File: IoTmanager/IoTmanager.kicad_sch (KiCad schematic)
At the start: 42 parts, among them J1 Program-connector, K1 ZC32F-012-HS3-copy, K2 ZC32F-012-HS3-copy, K3 ZC32F-012-HS3-copy, K4 ZC32F-012-HS3-copy, Q1 BC817, Q2 BC817, Q3 BC817, Q4 BC817, U1 NodeMCU_1.0_(ESP-12E), U2 ESP-12F, U3 TSOP23xx, U4 Mini360, U5 PJ-320A, U6 AMS1117-3.3

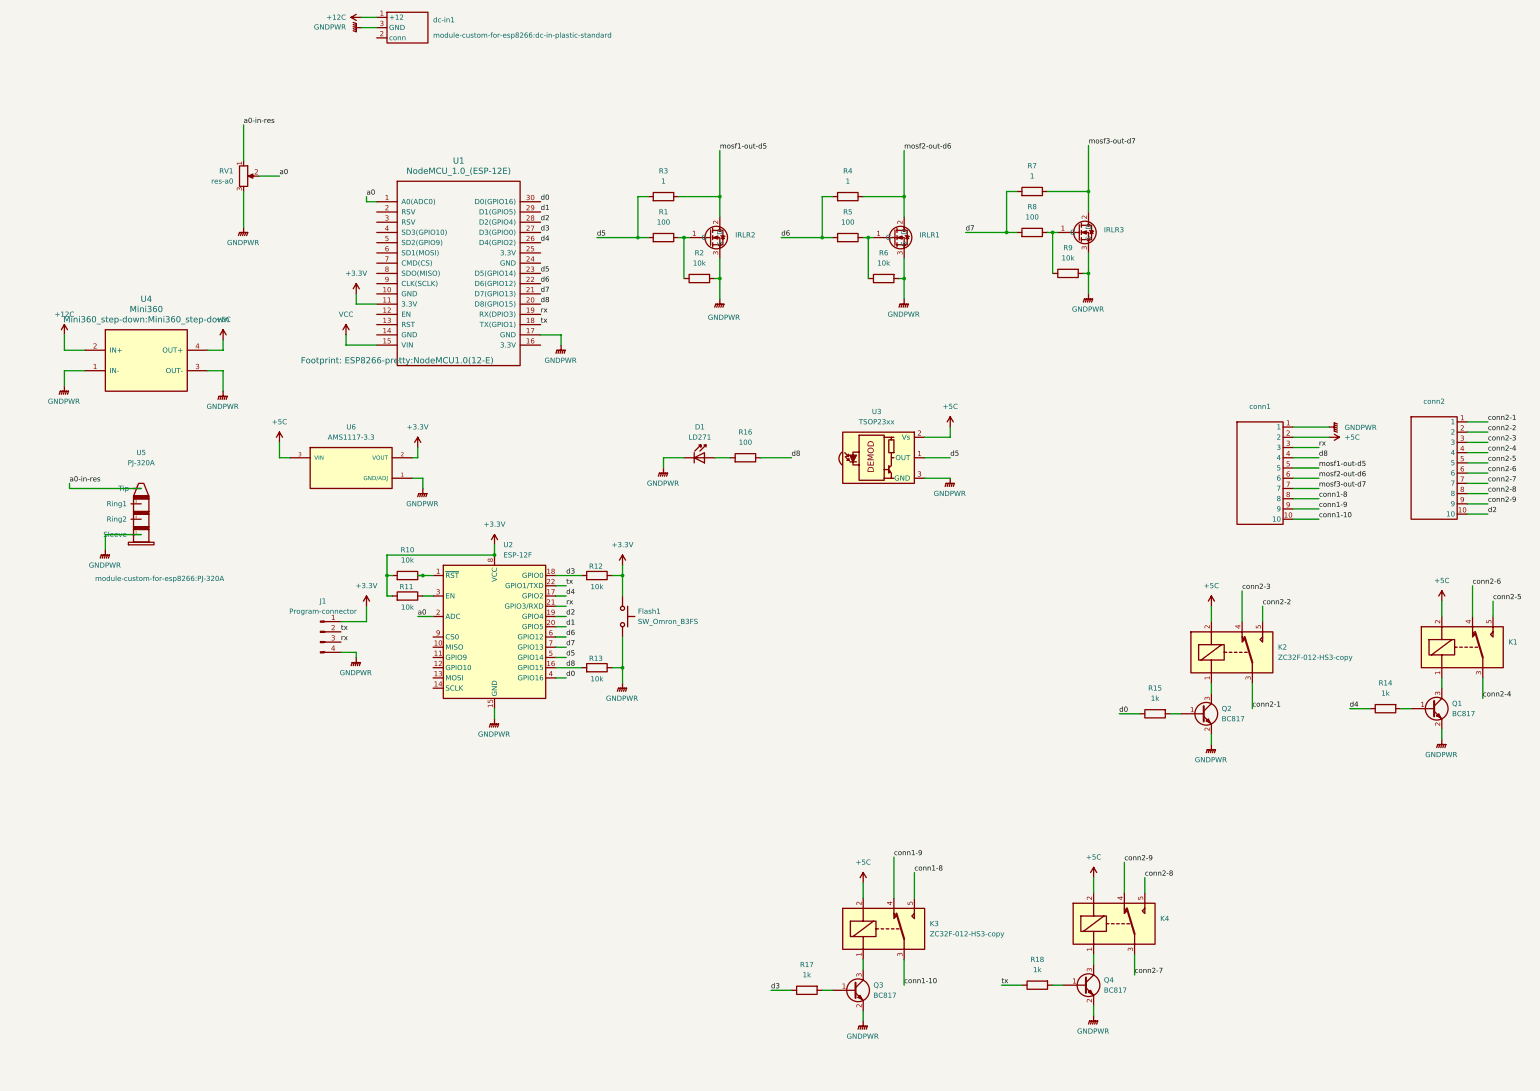
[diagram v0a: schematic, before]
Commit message: 123
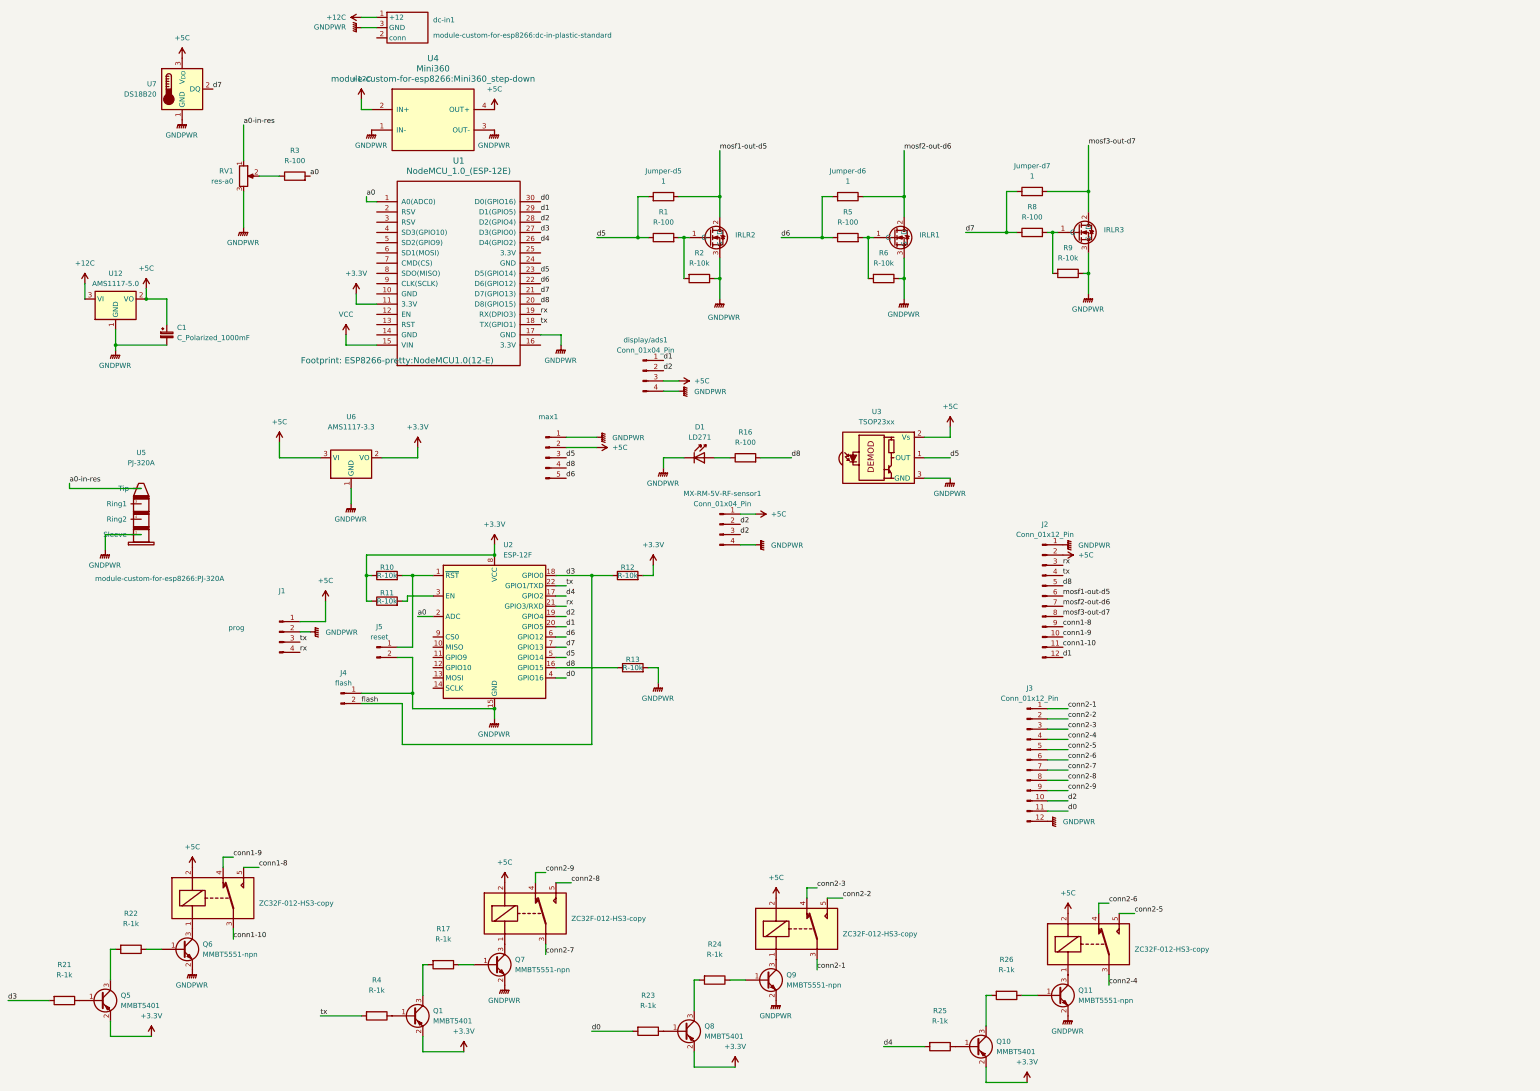
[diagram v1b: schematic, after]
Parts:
- removed Flash1: SW_Omron_B3FS, Button_Switch_SMD:SW_SPST_Omron_B3FS-100xP, symbol Switch:SW_Omron_B3FS
- removed K1, K2, K4: ZC32F-012-HS3-copy, module-custom-for-esp8266:ZC32F-012-HS3, symbol models:ZC32F-012-HS3-copy
- removed Q1, Q2, Q3, Q4: BC817, Package_TO_SOT_SMD:SOT-23, symbol Transistor_BJT:BC817
- removed R10: 10k, Resistor_SMD:R_0805_2012Metric, symbol resistor:R-base
- removed R14, R15, R17, R18: 1k, Resistor_SMD:R_0805_2012Metric, symbol resistor:R-base
- removed conn1, conn2: ~, module-custom-for-esp8266:connector-10, symbol models:CONNECTOR-10
- added C1: C_Polarized_1000mF, Capacitor_THT:CP_Radial_D10.0mm_P3.50mm, symbol resistor:C_Polarized_Small
- added J2, J3: Conn_01x12_Pin, module-custom-for-esp8266:connector-12-green-mini, symbol Connector:Conn_01x12_Pin
- added J4: flash, Connector_PinHeader_2.54mm:PinHeader_1x02_P2.54mm_Vertical, symbol Connector:Conn_01x02_Pin
- added J5: reset, Connector_PinHeader_2.54mm:PinHeader_1x02_P2.54mm_Vertical, symbol Connector:Conn_01x02_Pin
- added K5, K6, K7: ZC32F-012-HS3-copy, module-custom-for-esp8266:ZC32F-012-HS3, symbol models:ZC32F-012-HS3-copy
- added MX-RM-5V-RF-sensor1: Conn_01x04_Pin, module-custom-for-esp8266:RF_Receiver_433_MHz, symbol Connector:Conn_01x04_Pin
- added Q1, Q10, Q5, Q8: MMBT5401, Package_TO_SOT_SMD:SOT-23, symbol models:MMBT5401-pnp
- added Q11, Q6, Q7, Q9: MMBT5551-npn, Package_TO_SOT_SMD:SOT-23, symbol models:MMBT5551-npn
- added R10: R-10k, Resistor_SMD:R_0805_2012Metric, symbol models:R-10k
- added R17, R21, R22, R23, R24, R25, R26, R4: R-1k, Resistor_SMD:R_0805_2012Metric, symbol models:R-1k
- added R3: R-100, Resistor_SMD:R_0805_2012Metric, symbol models:R-100
- added U12: AMS1117-5.0, Package_TO_SOT_SMD:SOT-223-3_TabPin2, symbol Regulator_Linear:AMS1117-5.0
- added U7: DS18B20, Package_TO_SOT_THT:TO-92_Inline, symbol Sensor_Temperature:DS18B20
- added display/ads1: Conn_01x04_Pin, Connector_PinHeader_2.54mm:PinHeader_1x04_P2.54mm_Vertical, symbol Connector:Conn_01x04_Pin
- added max1: ~, Connector_PinHeader_2.54mm:PinHeader_1x05_P2.54mm_Vertical, symbol Connector:Conn_01x05_Pin
- IRLR1, IRLR2, IRLR3: footprint IRLR3103:DPAK229P990X239-4N -> Package_TO_SOT_SMD:TO-252-2
- J1: value Program-connector -> prog
- R1, R16, R5, R8: value 100 -> R-100; symbol resistor:R-base -> models:R-100; LCSC Part (none) -> C17408; Supplier (none) -> LCSCRef
- R11, R12, R13, R2, R6, R9: value 10k -> R-10k; symbol resistor:R-base -> models:R-10k; LCSC Part (none) -> C17414; Supplier (none) -> LCSCRef
- U3: footprint OptoDevice:Vishay_MINICAST-3Pin -> OptoDevice:Vishay_MOLD-3Pin
- U4: footprint Mini360_step-down:Mini360_step-down -> module-custom-for-esp8266:Mini360_step-down
- U5: LCSC Part (none) -> C2884926; Supplier (none) -> LCSCRef
- U6: LCSC Part (none) -> C6186; MAXIMUM_PACKAGE_HEIGHT 1.8 mm -> (none); Package SOT-223 Seeed Technology -> (none); Supplier (none) -> LCSCRef
- renumbered R3 to Jumper-d5, R4 to Jumper-d6, R7 to Jumper-d7
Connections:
- net +12C: now also U12.3 (VI)
- net +3.3V: now also Q1.2 (E), Q10.2 (E), Q5.2 (E), Q8.2 (E), R10.1; no longer J1.1 (Pin_1)
- net +5C: now also J1.1 (Pin_1), C1.1, J2.2 (Pin_2), K5.2, K6.2, K7.2, MX-RM-5V-RF-sensor1.1 (Pin_1), U12.2 (VO), U7.3 (V_{DD}), display/ads1.3 (Pin_3), max1.2 (Pin_2)
- net GNDPWR: now also J1.2 (Pin_2), C1.2, J2.1 (Pin_1), J3.12 (Pin_12), J4.1 (Pin_1), J5.2 (Pin_2), MX-RM-5V-RF-sensor1.4 (Pin_4), Q11.2 (E), Q6.2 (E), Q7.2 (E), Q9.2 (E), U12.1 (GND), U7.1 (GND), display/ads1.4 (Pin_4), max1.1 (Pin_1); no longer J1.4 (Pin_4)
- net a0: now also R3.2; no longer RV1.2
- net conn1-10: now also J2.11 (Pin_11)
- net conn1-8: now also J2.9 (Pin_9)
- net conn1-9: now also J2.10 (Pin_10)
- net conn2-1: now also J3.1 (Pin_1), K6.3
- net conn2-2: now also J3.2 (Pin_2), K6.5
- net conn2-3: now also J3.3 (Pin_3), K6.4
- net conn2-4: now also J3.4 (Pin_4), K7.3
- net conn2-5: now also J3.5 (Pin_5), K7.5
- net conn2-6: now also J3.6 (Pin_6), K7.4
- net conn2-7: now also J3.7 (Pin_7), K5.3
- net conn2-8: now also J3.8 (Pin_8), K5.5
- net conn2-9: now also J3.9 (Pin_9), K5.4
- net d0: now also J3.11 (Pin_11), R23.2
- net d1: now also J2.12 (Pin_12), display/ads1.1 (Pin_1)
- net d2: now also J3.10 (Pin_10), MX-RM-5V-RF-sensor1.2 (Pin_2), MX-RM-5V-RF-sensor1.3 (Pin_3), display/ads1.2 (Pin_2)
- net d3: now also J4.2 (Pin_2), R21.2
- net d4: now also R25.2
- net d5: now also max1.3 (Pin_3)
- net d6: now also max1.5 (Pin_5)
- net d7: now also U7.2 (DQ)
- net d8: now also J2.5 (Pin_5), max1.4 (Pin_4)
- net mosf1-out-d5: now also J2.6 (Pin_6)
- net mosf2-out-d6: now also J2.7 (Pin_7)
- net mosf3-out-d7: now also J2.8 (Pin_8)
- net rx: now also J1.4 (Pin_4), J2.3 (Pin_3); no longer J1.3 (Pin_3)
- net tx: now also J1.3 (Pin_3), J2.4 (Pin_4), R4.2; no longer J1.2 (Pin_2)
- net at K3.1: now also Q6.3 (C)
- net at U2.1 (~{RST}): now also J5.1 (Pin_1), R10.2
- new net: Q5.1 (B), R21.1
- new net: Q9.1 (B), R24.1
- new net: K6.1, Q9.3 (C)
- new net: K7.1, Q11.3 (C)
- new net: K5.1, Q7.3 (C)
- new net: R3.1, RV1.2
- new net: Q5.3 (C), R22.2
- new net: Q6.1 (B), R22.1
- new net: Q11.1 (B), R26.1
- new net: Q10.3 (C), R26.2
- new net: Q8.3 (C), R24.2
- new net: Q7.1 (B), R17.1
- new net: Q1.3 (C), R17.2
- new net: Q10.1 (B), R25.1
- new net: Q8.1 (B), R23.1
- new net: Q1.1 (B), R4.1
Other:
- moved on the sheet: J1, R11, R12, R13
